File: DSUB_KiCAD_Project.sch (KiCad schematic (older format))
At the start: 6 parts, among them J1 XT60-M, J2 XT60-M, J3 XT60-M, J4 XT60-M, J5 XT60-M, J6 Barrel_Jack

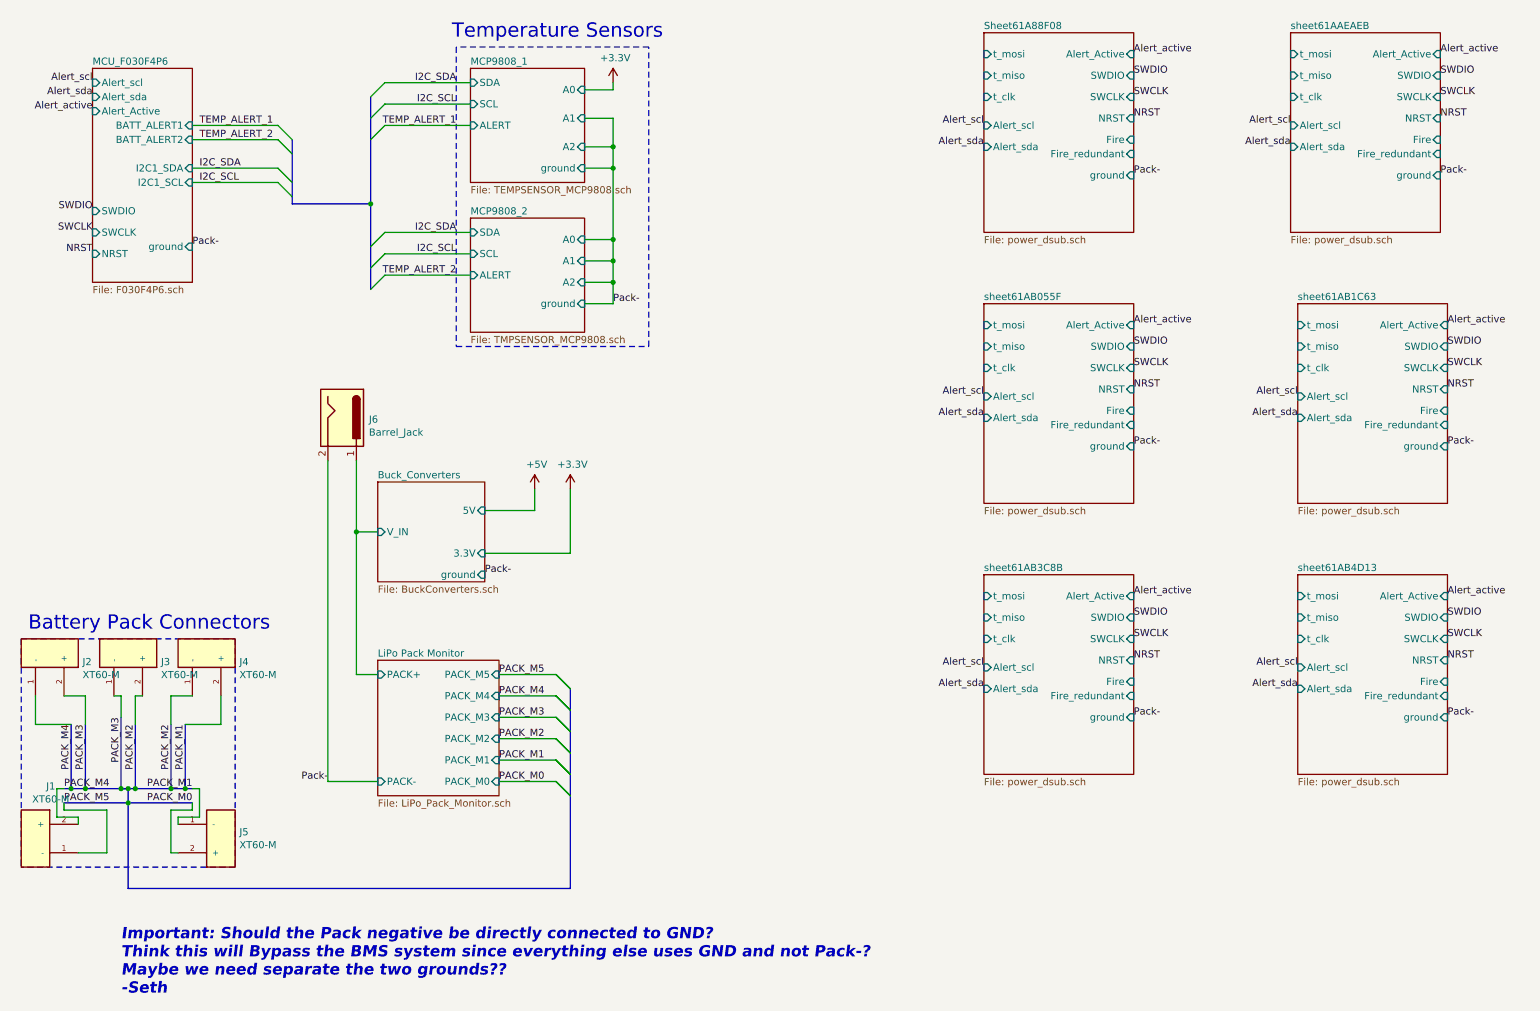
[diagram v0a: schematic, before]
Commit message: Pcb made
actually made the pcb
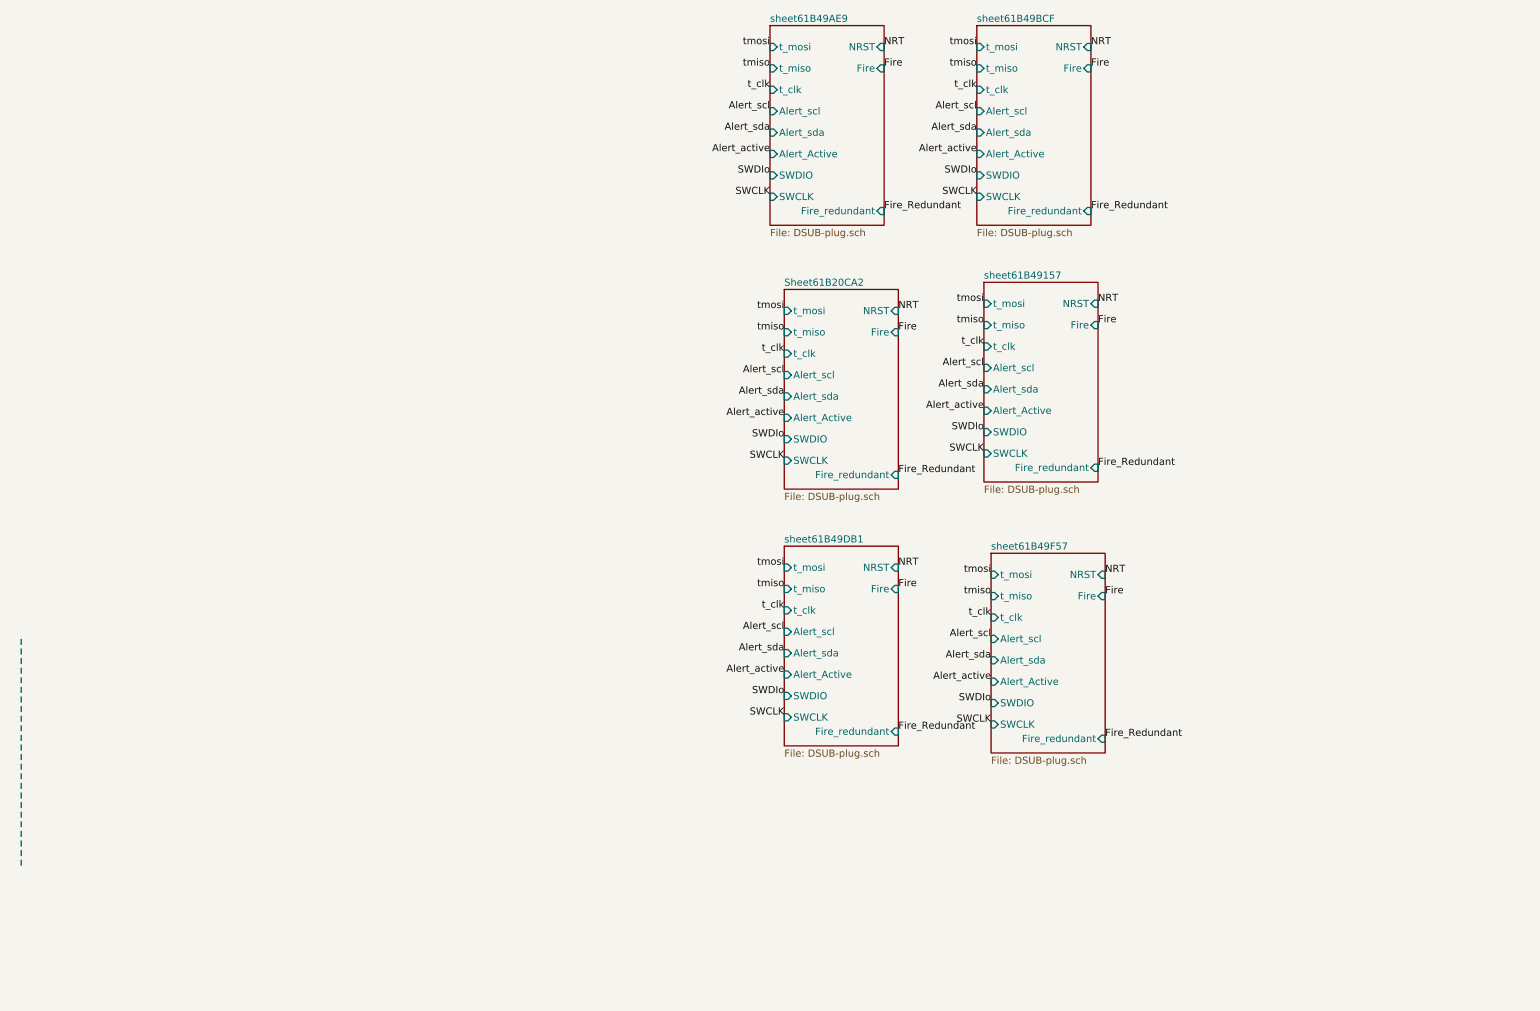
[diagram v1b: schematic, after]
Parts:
- removed J1, J2, J3, J4, J5: XT60-M, XT60-M:AMASS_XT60-M, symbol XT60-M:XT60-M
- removed J6: Barrel_Jack, Connector_BarrelJack:BarrelJack_CUI_PJ-036AH-SMT_Horizontal, symbol Connector:Barrel_Jack
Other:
- note removed: "Battery Pack Connectors"
- note removed: "Important: Should the Pack negative be directly connected to GND?\nThink this will Bypass the BMS system since everything else uses GND and not Pack-?\nMaybe we need separate the two grounds??\n-Seth"
- note removed: "Temperature Sensors"
